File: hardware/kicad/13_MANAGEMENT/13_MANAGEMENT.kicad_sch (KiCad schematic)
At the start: 1 part

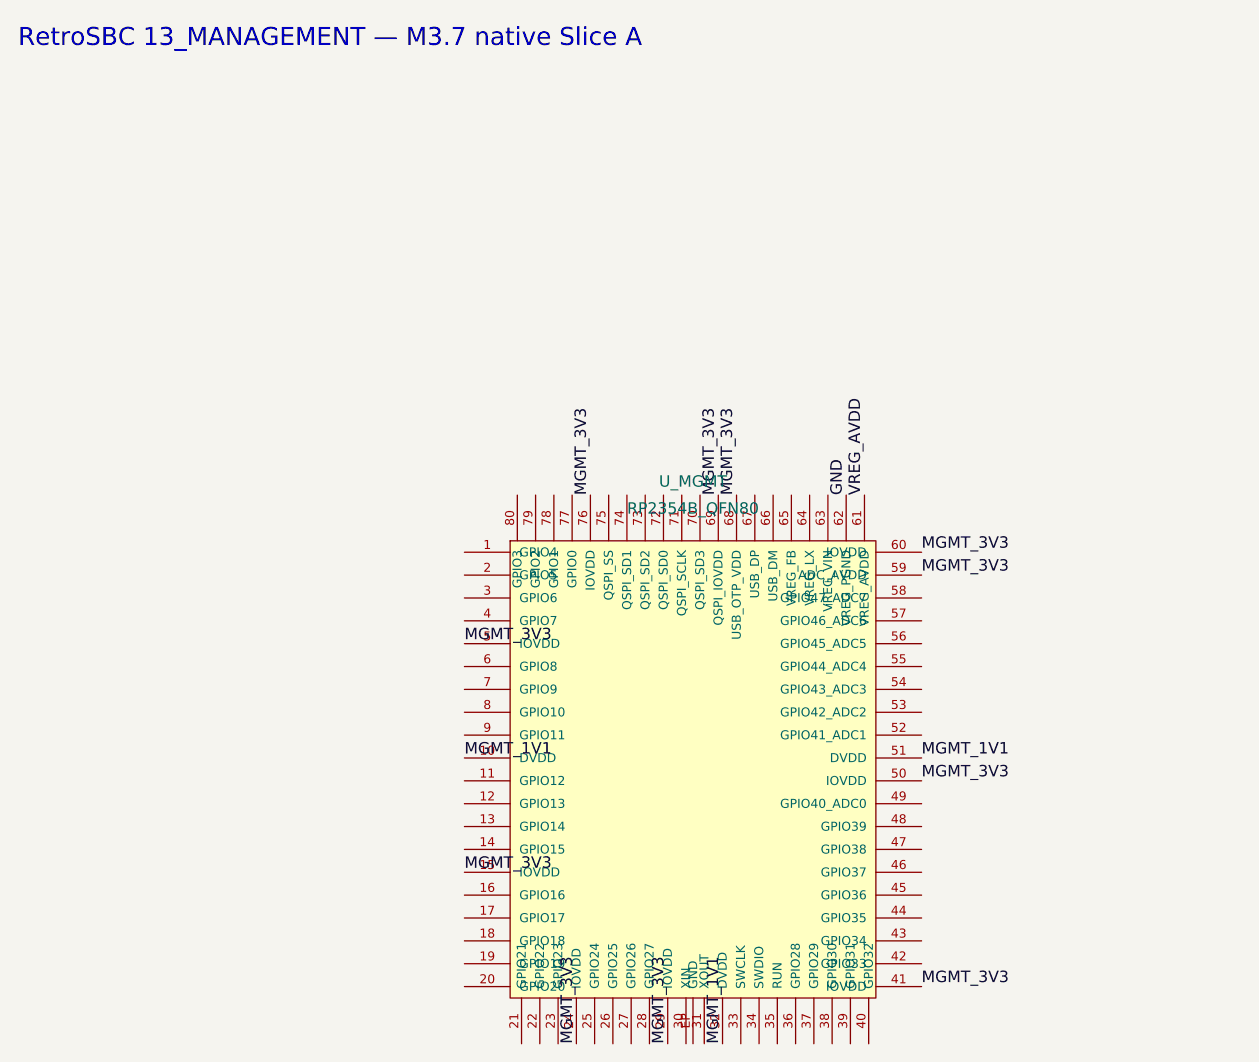
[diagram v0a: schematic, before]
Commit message: M3.7: restore native Slice A passive instances
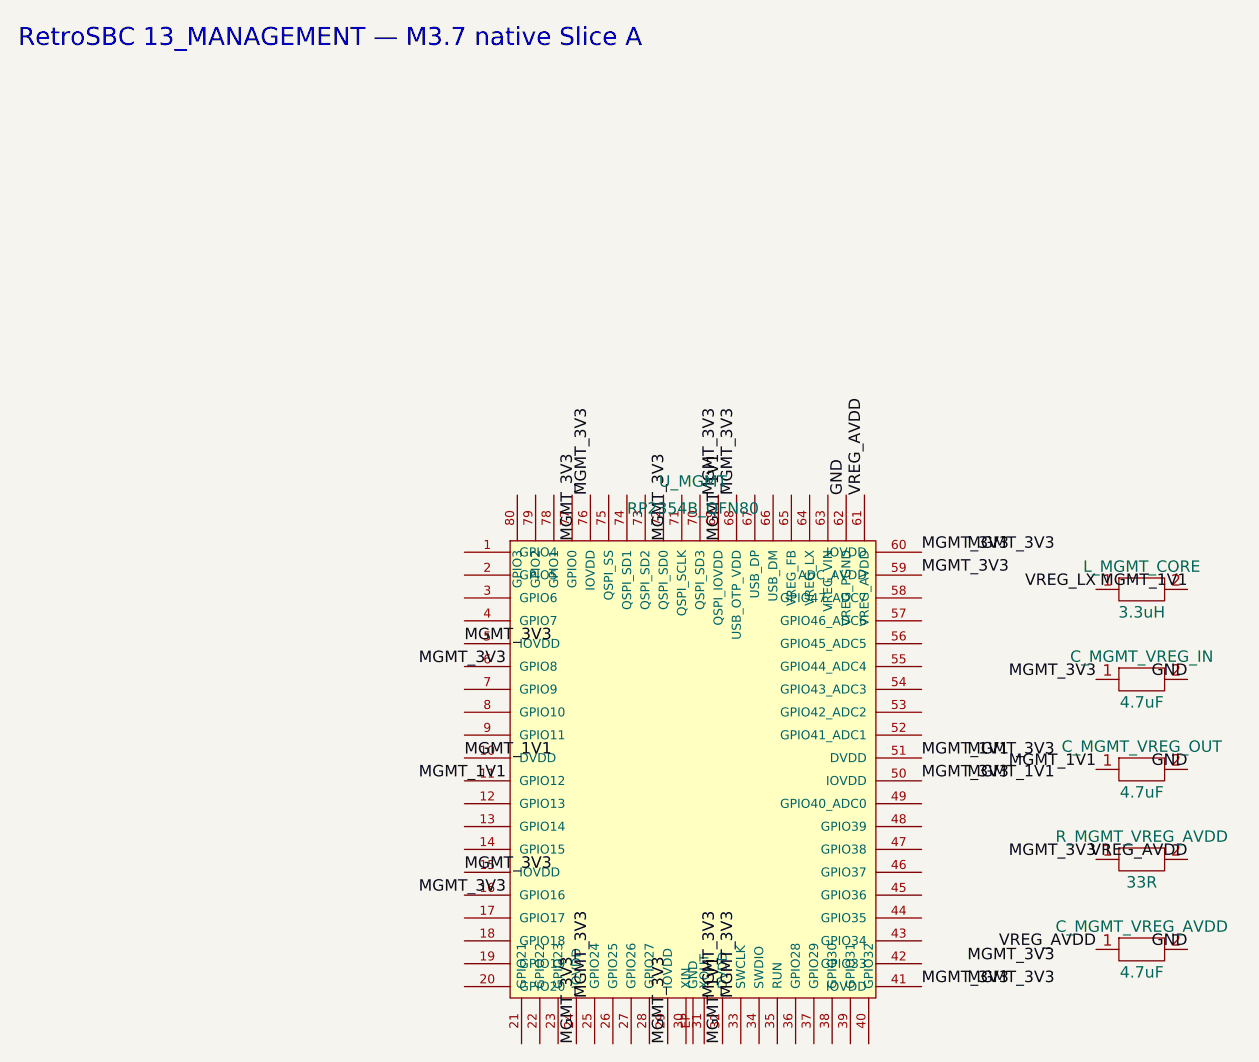
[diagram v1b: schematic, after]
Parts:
- added C_MGMT_VREG_AVDD, C_MGMT_VREG_IN, C_MGMT_VREG_OUT: 4.7uF, symbol RetroSBC-management:C_LOCAL
- added L_MGMT_CORE: 3.3uH, symbol RetroSBC-management:L_LOCAL
- added R_MGMT_VREG_AVDD: 33R, symbol RetroSBC-management:R_LOCAL
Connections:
- net GND: now also C_MGMT_VREG_AVDD.2, C_MGMT_VREG_IN.2, C_MGMT_VREG_OUT.2
- net MGMT_1V1: now also C_MGMT_VREG_OUT.1, L_MGMT_CORE.2
- net MGMT_3V3: now also C_MGMT_VREG_IN.1, R_MGMT_VREG_AVDD.1
- net VREG_AVDD: now also C_MGMT_VREG_AVDD.1, R_MGMT_VREG_AVDD.2
- new net VREG_LX: L_MGMT_CORE.1
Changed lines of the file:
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@@
     ))
   )
+  (symbol (lib_id "RetroSBC-management:L_LOCAL") (at 149.86 80 0) (unit 1)
+    (exclude_from_sim no) (in_bom yes) (on_board yes)
+    (property "Reference" "L_MGMT_CORE" (at 149.86 77.46 0) (effects (font (size 1.27 1.27))))
+    (property "Value" "3.3uH" (at 149.86 82.54 0) (effects (font (size 1.27 1.27))))
+    (property "Footprint" "" (at 149.86 80 0) (effects (font (size 1.27 1.27)) hide))
+    (property "Datasheet" "" (at 149.86 80 0) (effects (font (size 1.27 1.27)) hide))
+    (property "Description" "RetroSBC local passive" (at 149.86 80 0) (effects (font (size 1.27 1.27)) hide))
+    (pin "1")
+    (pin "2")
+    (instances (project "RetroSBC-13-MANAGEMENT" (path "/7a5d3d51-9e2f-4d31-b7cb-9fbd10b8c301/21111111-1111-4111-8111-222222222222" (reference "L_MGMT_CORE") (unit 1))))
+  )
+  (label "VREG_LX" (at 144.78 80 0) (effects (font (size 1.27 1.27)) (justify right bottom)))
+  (label "MGMT_1V1" (at 154.94 80 180) (effects (font (size 1.27 1.27)) (justify right bottom)))
+  (symbol (lib_id "RetroSBC-management:C_LOCAL") (at 149.86 90 0) (unit 1)
+    (exclude_from_sim no) (in_bom yes) (on_board yes)
+    (property "Reference" "C_MGMT_VREG_IN" (at 149.86 87.46 0) (effects (font (size 1.27 1.27))))
+    (property "Value" "4.7uF" (at 149.86 92.54 0) (effects (font (size 1.27 1.27))))
+    (property "Footprint" "" (at 149.86 90 0) (effects (font (size 1.27 1.27)) hide))
+    (property "Datasheet" "" (at 149.86 90 0) (effects (font (size 1.27 1.27)) hide))
+    (property "Description" "RetroSBC local passive" (at 149.86 90 0) (effects (font (size 1.27 1.27)) hide))
+    (pin "1")
+    (pin "2")
+    (instances (project "RetroSBC-13-MANAGEMENT" (path "/7a5d3d51-9e2f-4d31-b7cb-9fbd10b8c301/31111111-1111-4111-8111-333333333333" (reference "C_MGMT_VREG_IN") (unit 1))))
+  )
+  (label "MGMT_3V3" (at 144.78 90 0) (effects (font (size 1.27 1.27)) (justify right bottom)))
+  (label "GND" (at 154.94 90 180) (effects (font (size 1.27 1.27)) (justify right bottom)))
+  (symbol (lib_id "RetroSBC-management:C_LOCAL") (at 149.86 100 0) (unit 1)
+    (exclude_from_sim no) (in_bom yes) (on_board yes)
+    (property "Reference" "C_MGMT_VREG_OUT" (at 149.86 97.46 0) (effects (font (size 1.27 1.27))))
+    (property "Value" "4.7uF" (at 149.86 102.54 0) (effects (font (size 1.27 1.27))))
+    (property "Footprint" "" (at 149.86 100 0) (effects (font (size 1.27 1.27)) hide))
+    (property "Datasheet" "" (at 149.86 100 0) (effects (font (size 1.27 1.27)) hide))
+    (property "Description" "RetroSBC local passive" (at 149.86 100 0) (effects (font (size 1.27 1.27)) hide))
+    (pin "1")
+    (pin "2")
+    (instances (project "RetroSBC-13-MANAGEMENT" (path "/7a5d3d51-9e2f-4d31-b7cb-9fbd10b8c301/41111111-1111-4111-8111-444444444444" (reference "C_MGMT_VREG_OUT") (unit 1))))
+  )
+  (label "MGMT_1V1" (at 144.78 100 0) (effects (font (size 1.27 1.27)) (justify right bottom)))
+  (label "GND" (at 154.94 100 180) (effects (font (size 1.27 1.27)) (justify right bottom)))
+  (symbol (lib_id "RetroSBC-management:R_LOCAL") (at 149.86 110 0) (unit 1)
+    (exclude_from_sim no) (in_bom yes) (on_board yes)
+    (property "Reference" "R_MGMT_VREG_AVDD" (at 149.86 107.46 0) (effects (font (size 1.27 1.27))))
+    (property "Value" "33R" (at 149.86 112.54 0) (effects (font (size 1.27 1.27))))
+    (property "Footprint" "" (at 149.86 110 0) (effects (font (size 1.27 1.27)) hide))
+    (property "Datasheet" "" (at 149.86 110 0) (effects (font (size 1.27 1.27)) hide))
+    (property "Description" "RetroSBC local passive" (at 149.86 110 0) (effects (font (size 1.27 1.27)) hide))
+    (pin "1")
+    (pin "2")
+    (instances (project "RetroSBC-13-MANAGEMENT" (path "/7a5d3d51-9e2f-4d31-b7cb-9fbd10b8c301/51111111-1111-4111-8111-555555555555" (reference "R_MGMT_VREG_AVDD") (unit 1))))
+  )
+  (label "MGMT_3V3" (at 144.78 110 0) (effects (font (size 1.27 1.27)) (justify right bottom)))
+  (label "VREG_AVDD" (at 154.94 110 180) (effects (font (size 1.27 1.27)) (justify right bottom)))
+  (symbol (lib_id "RetroSBC-management:C_LOCAL") (at 149.86 120 0) (unit 1)
+    (exclude_from_sim no) (in_bom yes) (on_board yes)
+    (property "Reference" "C_MGMT_VREG_AVDD" (at 149.86 117.46 0) (effects (font (size 1.27 1.27))))
+    (property "Value" "4.7uF" (at 149.86 122.54 0) (effects (font (size 1.27 1.27))))
+    (property "Footprint" "" (at 149.86 120 0) (effects (font (size 1.27 1.27)) hide))
+    (property "Datasheet" "" (at 149.86 120 0) (effects (font (size 1.27 1.27)) hide))
+    (property "Description" "RetroSBC local passive" (at 149.86 120 0) (effects (font (size 1.27 1.27)) hide))
+    (pin "1")
+    (pin "2")
+    (instances (project "RetroSBC-13-MANAGEMENT" (path "/7a5d3d51-9e2f-4d31-b7cb-9fbd10b8c301/61111111-1111-4111-8111-666666666666" (reference "C_MGMT_VREG_AVDD") (unit 1))))
+  )
+  (label "VREG_AVDD" (at 144.78 120 0) (effects (font (size 1.27 1.27)) (justify right bottom)))
+  (label "GND" (at 154.94 120 180) (effects (font (size 1.27 1.27)) (justify right bottom)))
+  (label "MGMT_3V3" (at 69.52000000000001 113.97 0)
+    (effects (font (size 1.27 1.27)) (justify left bottom))
+)
+  (label "MGMT_1V1" (at 69.52000000000001 101.27 0)
+    (effects (font (size 1.27 1.27)) (justify left bottom))
+)
+  (label "MGMT_3V3" (at 69.52000000000001 88.57 0)
+    (effects (font (size 1.27 1.27)) (justify left bottom))
+)
+  (label "MGMT_3V3" (at 87.03999999999999 74.6 90)
+    (effects (font (size 1.27 1.27)) (justify left bottom))
+)
+  (label "MGMT_3V3" (at 97.19 74.6 90)
+    (effects (font (size 1.27 1.27)) (justify left bottom))
+)
+  (label "MGMT_1V1" (at 103.28 74.6 90)
+    (effects (font (size 1.27 1.27)) (justify left bottom))
+)
+  (label "MGMT_3V3" (at 130.48 75.87 180)
+    (effects (font (size 1.27 1.27)) (justify left bottom))
+)
+  (label "MGMT_3V3" (at 130.48 98.73 180)
+    (effects (font (size 1.27 1.27)) (justify left bottom))
+)
+  (label "MGMT_1V1" (at 130.48 101.27 180)
+    (effects (font (size 1.27 1.27)) (justify left bottom))
+)
+  (label "MGMT_3V3" (at 130.48 121.59 180)
+    (effects (font (size 1.27 1.27)) (justify left bottom))
+)
+  (label "MGMT_3V3" (at 130.48 124.13 180)
+    (effects (font (size 1.27 1.27)) (justify left bottom))
+)
+  (label "MGMT_3V3" (at 104.84 125.4 270)
+    (effects (font (size 1.27 1.27)) (justify left bottom))
+)
+  (label "MGMT_3V3" (at 102.81 125.4 270)
+    (effects (font (size 1.27 1.27)) (justify left bottom))
+)
+  (label "MGMT_3V3" (at 88.60000000000001 125.4 270)
+    (effects (font (size 1.27 1.27)) (justify left bottom))
+)
   (label "VREG_AVDD" (at 119.05 69.52 90)
     (effects (font (size 1.27 1.27)) (justify left bottom))
